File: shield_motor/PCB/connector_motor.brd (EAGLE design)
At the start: 68.6 x 53.3 mm, 14 parts

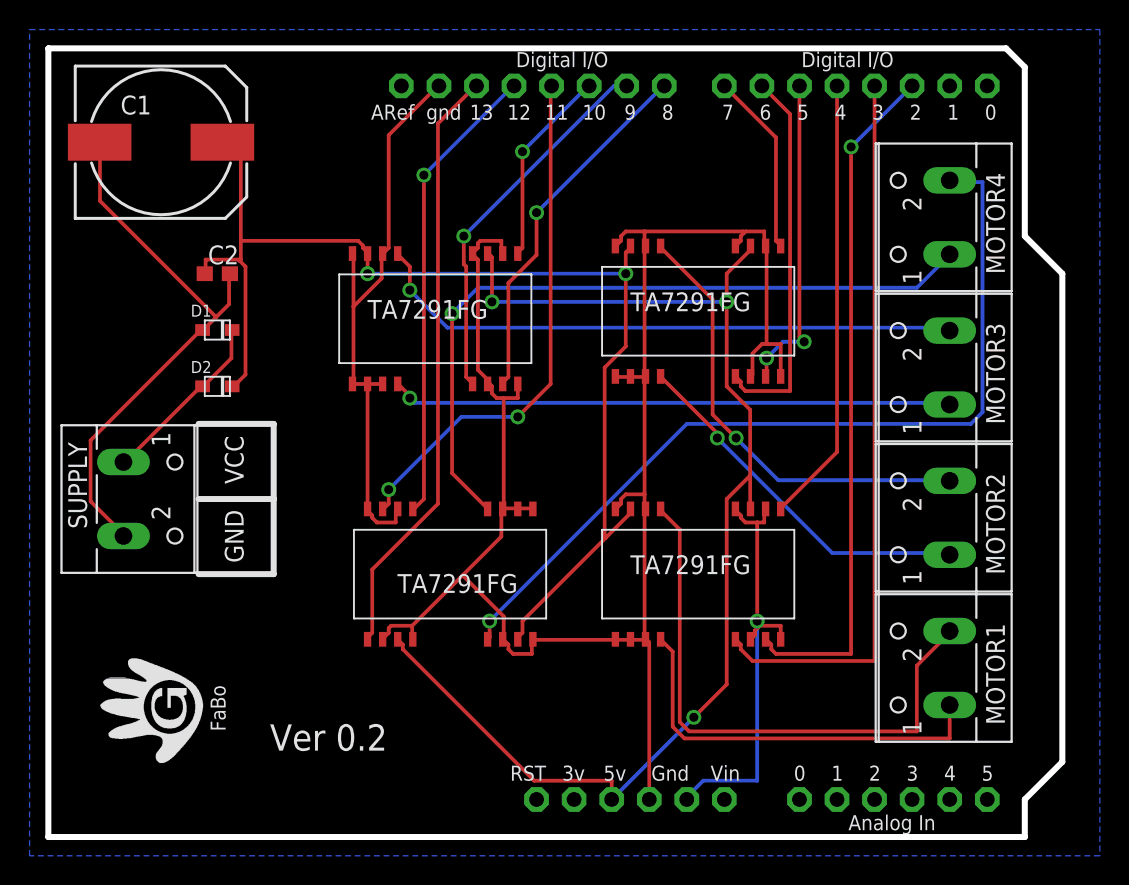
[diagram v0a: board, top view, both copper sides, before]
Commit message: Modified brick
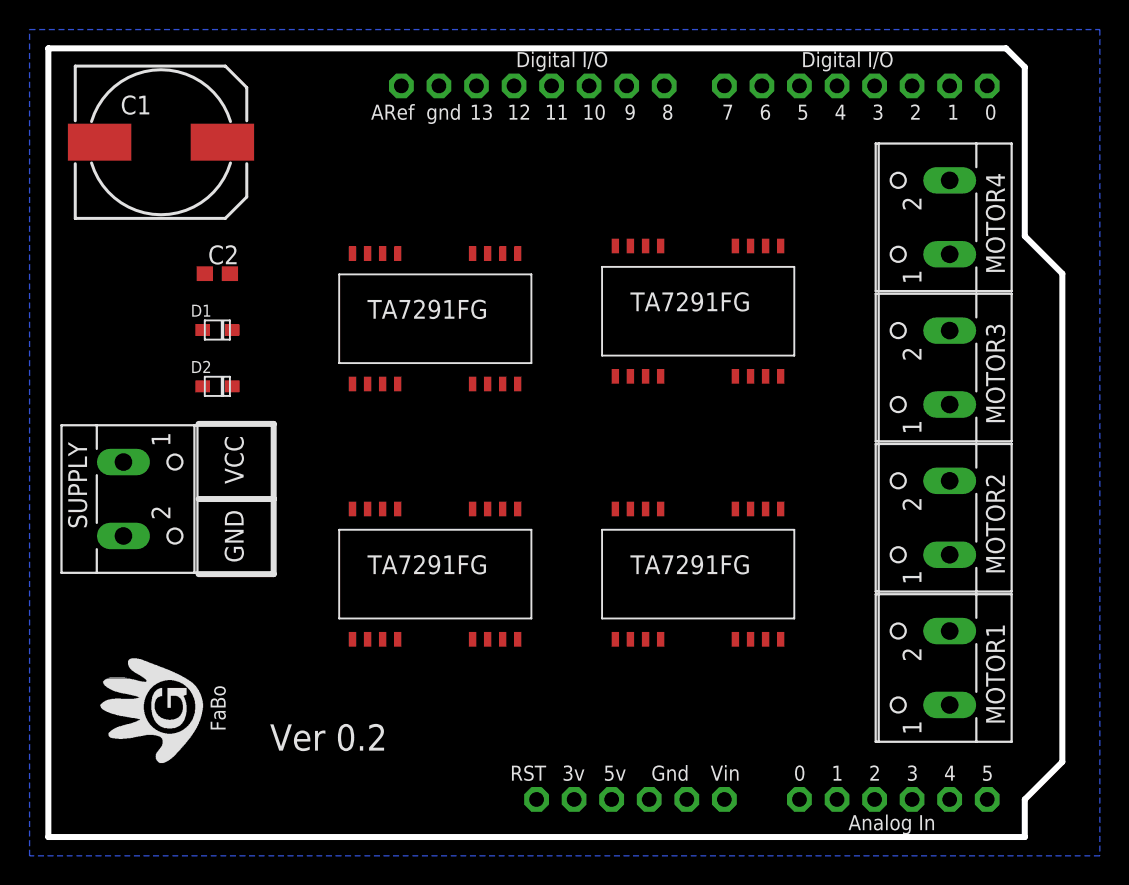
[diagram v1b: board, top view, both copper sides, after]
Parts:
- turned U$5 to 0 degrees
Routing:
- net GND: track 233.5 -> 0.00 mm, vias 1 -> 0
- net VCC: track 84.1 -> 0.00 mm, vias 3 -> 0
- net M_VCC: track 81.4 -> 0.00 mm, vias 2 -> 0
- net M4_OUT2: track 58.4 -> 0.00 mm, vias 1 -> 0
- net M4_OUT1: track 49.5 -> 0.00 mm, vias 1 -> 0
- net M1_REF: track 49.1 -> 0.00 mm
- net M1_IN1: track 46.5 -> 0.00 mm, vias 1 -> 0
- net M4_IN2: track 40.5 -> 0.00 mm
- net M3_OUT2: track 40.5 -> 0.00 mm, vias 1 -> 0
- net M1_OUT2: track 38.9 -> 0.00 mm
- net M3_OUT1: track 38.1 -> 0.00 mm, vias 1 -> 0
- net M4_IN1: track 35.6 -> 0.00 mm, vias 2 -> 0
- net M4_REF: track 31.5 -> 0.00 mm, vias 1 -> 0
- net M2_OUT2: track 30.8 -> 0.00 mm, vias 1 -> 0
- net M1_IN2: track 30.2 -> 0.00 mm
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
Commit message: Update for elect
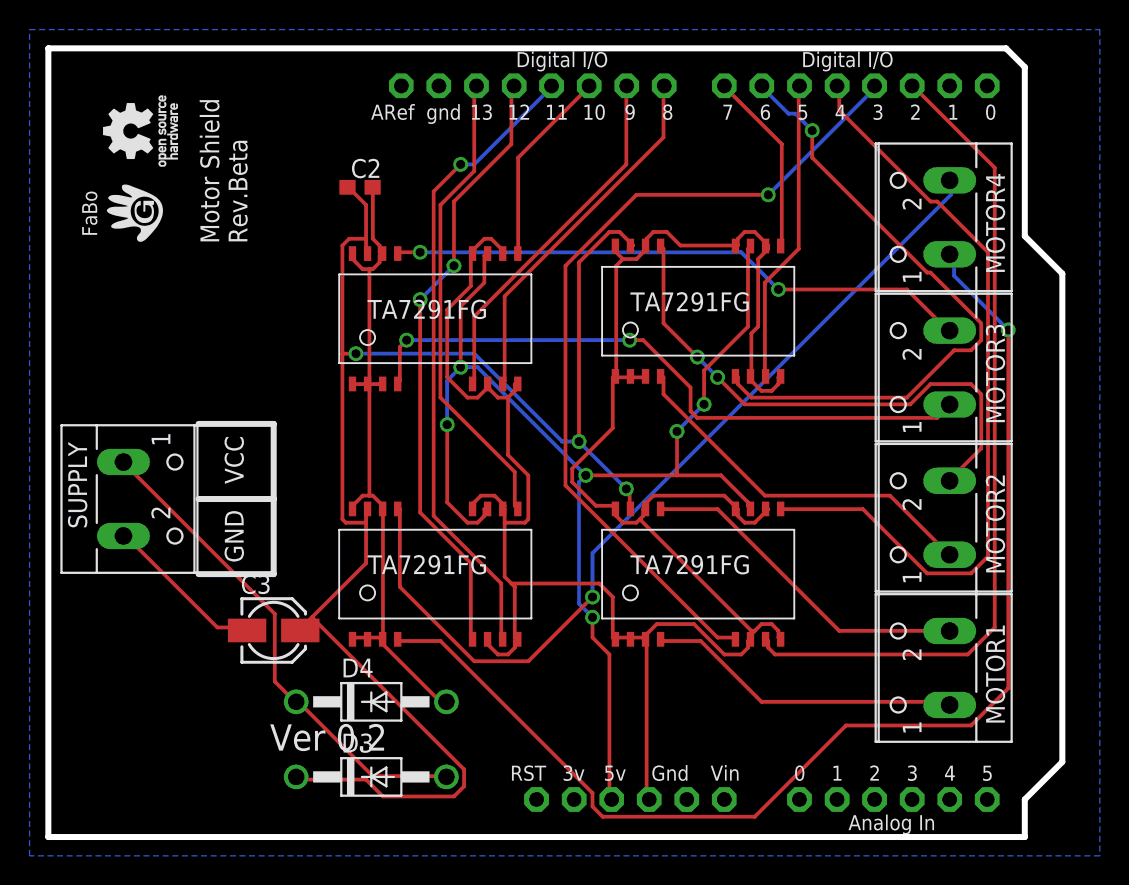
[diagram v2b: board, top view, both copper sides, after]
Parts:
- removed C1: 100uf, adafruit:150CLZ-1014
- removed D1: (no value), adafruit:SOD-323F
- removed D2: 1N4148, adafruit:SOD-323F
- added C3: 100uf, resistor:153CLV-0405
- added D3, D4: 1N4004, diode:DO41-10
- added U$6: (no value), gclue:LOGO_OSHW_T_M
- added U$7: (no value), gclue:LOGO_FABO_M
- moved C2 11.3 mm to (21.1, 43.9)
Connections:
- net GND: now also C3.-, D4.A; no longer C1.-, D1.A
- net M_VCC: now also C3.+, D3.C; no longer C1.+, D2.C
- net N$1: now also D3.A, D4.C; no longer D1.C, D2.A
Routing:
- net GND: track 0.00 -> 212.1 mm
- net M_VCC: track 0.00 -> 106.7 mm, vias 0 -> 3
- net VCC: track 0.00 -> 86.2 mm, vias 0 -> 6
- net M4_OUT1: track 0.00 -> 81.4 mm, vias 0 -> 1
- net M4_OUT2: track 0.00 -> 60.6 mm, vias 0 -> 1
- net M1_REF: track 0.00 -> 56.9 mm, vias 0 -> 1
- net M1_IN1: track 0.00 -> 55.9 mm
- net M1_IN2: track 0.00 -> 52.7 mm
- net M3_OUT1: track 0.00 -> 43.4 mm, vias 0 -> 2
- net M4_IN1: track 0.00 -> 43.2 mm, vias 0 -> 1
- net M2_REF: track 0.00 -> 42.8 mm, vias 0 -> 1
- net M4_REF: track 0.00 -> 41.6 mm, vias 0 -> 2
- net M3_OUT2: track 0.00 -> 39.5 mm, vias 0 -> 2
- net M2_OUT2: track 0.00 -> 36.6 mm, vias 0 -> 2
- net N$1: track 0.00 -> 33.3 mm
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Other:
- board text added: "Motor Shield Rev.Beta"
- board text removed: "FaBo"
